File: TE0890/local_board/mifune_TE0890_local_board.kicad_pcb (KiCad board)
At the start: 2 copper layers, 139.7 x 120.7 mm, 76 parts, among them J1 Conn_01x01, J10 Conn_01x01, J11 Conn_01x01, J12 Conn_01x01, J13 1734035-1, J14 Conn_01x01, J15 Conn_01x01, J2 Conn_01x01, J3 Conn_01x01, J4 Conn_01x01, J5 Conn_01x01, J6 Conn_01x01, J7 Conn_01x01, J8 Conn_01x01, J9 Conn_01x01, U1 TE0890_80P, U2 TE0890_JTAG, U3 TE0790_Std, U4 TE0890_FTDI

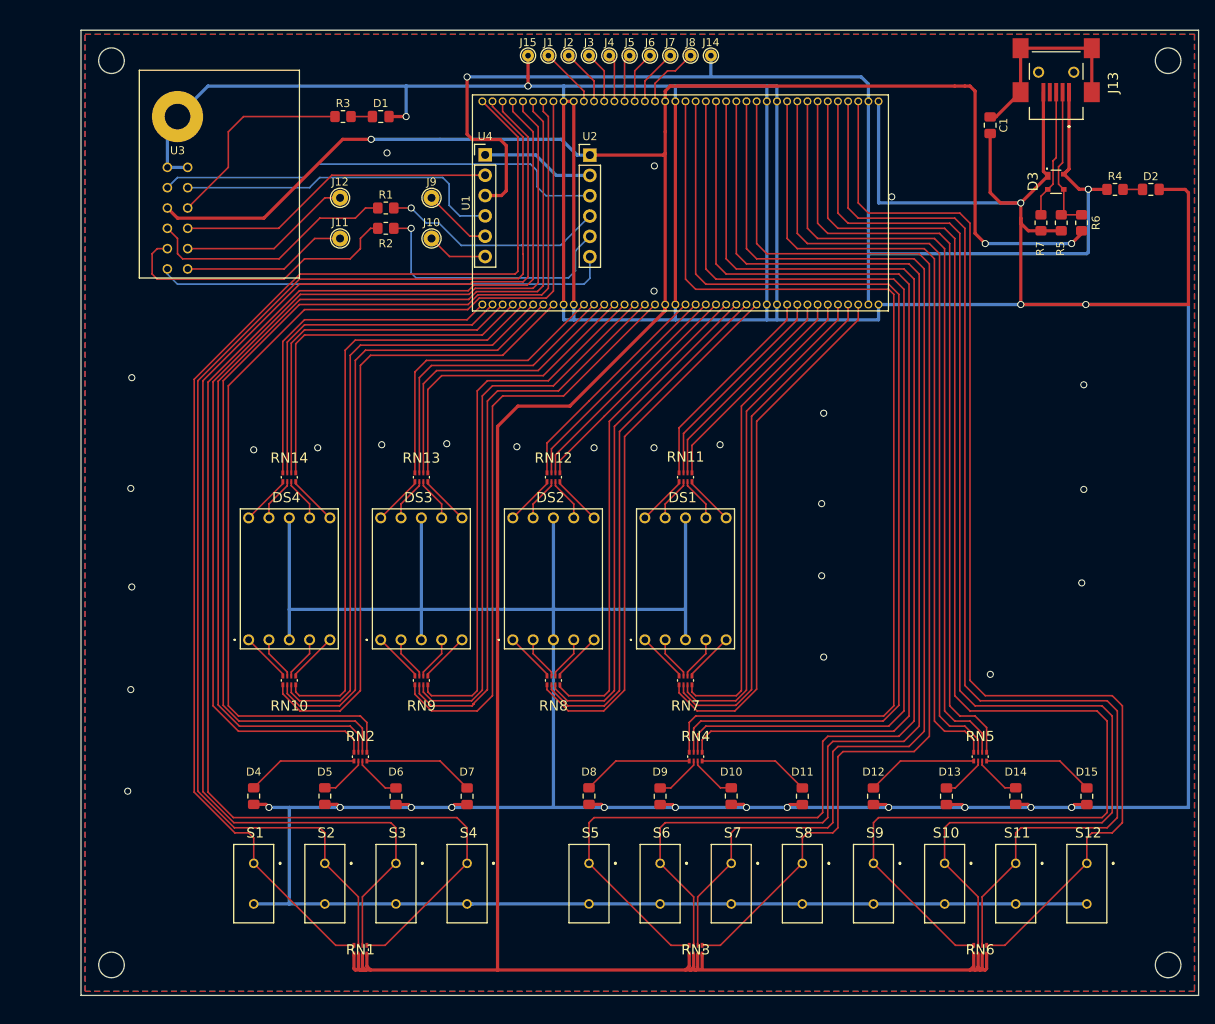
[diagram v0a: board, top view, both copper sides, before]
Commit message: local board rev.1.0 work in progress
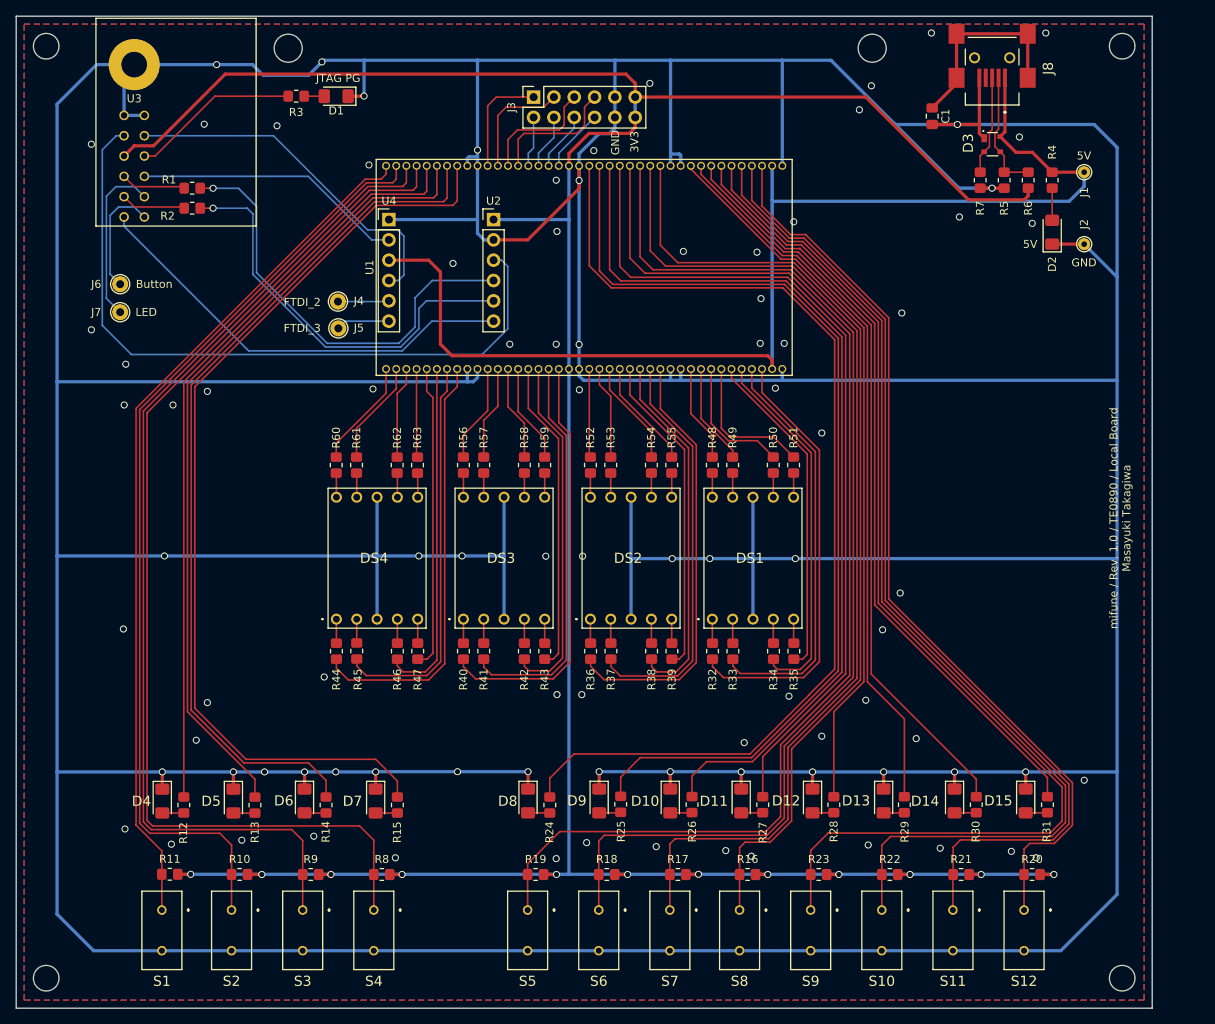
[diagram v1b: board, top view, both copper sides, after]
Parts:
- removed J10, J11, J12, J9: Conn_01x01, TestPoint:TestPoint_THTPad_D2.0mm_Drill1.0mm
- removed J13: 1734035-1, LibraryLoader:17340351
- removed J14, J15: Conn_01x01, TestPoint:TestPoint_THTPad_D1.5mm_Drill0.7mm
- removed RN1, RN10, RN11, RN12, RN13, RN14, RN2, RN3, RN4, RN5, RN6, RN7, RN8, RN9: EXB-N8V820JX, LibraryLoader:EXBN8V510JX
- added H5: MountingHole, MountingHole:MountingHole_3.5mm, F.Cu at (137.0, 34.0)
- added H6: MountingHole, MountingHole:MountingHole_3.5mm, F.Cu at (64.0, 34.0)
- added R10: 10k, Resistor_SMD:R_0805_2012Metric_Pad1.20x1.40mm_HandSolder, F.Cu at (57.9, 137.3)
- added R11: 10k, Resistor_SMD:R_0805_2012Metric_Pad1.20x1.40mm_HandSolder, F.Cu at (49.2, 137.3)
- added R12: 120, Resistor_SMD:R_0805_2012Metric_Pad1.20x1.40mm_HandSolder, F.Cu at (51.0, 128.6)
- added R13: 120, Resistor_SMD:R_0805_2012Metric_Pad1.20x1.40mm_HandSolder, F.Cu at (59.8, 128.6)
- added R14: 120, Resistor_SMD:R_0805_2012Metric_Pad1.20x1.40mm_HandSolder, F.Cu at (68.7, 128.6)
- added R15: 120, Resistor_SMD:R_0805_2012Metric_Pad1.20x1.40mm_HandSolder, F.Cu at (77.6, 128.6)
- added R16: 10k, Resistor_SMD:R_0805_2012Metric_Pad1.20x1.40mm_HandSolder, F.Cu at (121.4, 137.3)
- added R17: 10k, Resistor_SMD:R_0805_2012Metric_Pad1.20x1.40mm_HandSolder, F.Cu at (112.7, 137.3)
- added R18: 10k, Resistor_SMD:R_0805_2012Metric_Pad1.20x1.40mm_HandSolder, F.Cu at (103.8, 137.3)
- added R19: 10k, Resistor_SMD:R_0805_2012Metric_Pad1.20x1.40mm_HandSolder, F.Cu at (94.9, 137.3)
- added R20: 10k, Resistor_SMD:R_0805_2012Metric_Pad1.20x1.40mm_HandSolder, F.Cu at (157.0, 137.3)
- added R21: 10k, Resistor_SMD:R_0805_2012Metric_Pad1.20x1.40mm_HandSolder, F.Cu at (148.1, 137.3)
- added R22: 10k, Resistor_SMD:R_0805_2012Metric_Pad1.20x1.40mm_HandSolder, F.Cu at (139.2, 137.3)
- added R23: 10k, Resistor_SMD:R_0805_2012Metric_Pad1.20x1.40mm_HandSolder, F.Cu at (130.3, 137.3)
- added R24: 120, Resistor_SMD:R_0805_2012Metric_Pad1.20x1.40mm_HandSolder, F.Cu at (96.7, 128.6)
- added R25: 120, Resistor_SMD:R_0805_2012Metric_Pad1.20x1.40mm_HandSolder, F.Cu at (105.6, 128.5)
- added R26: 120, Resistor_SMD:R_0805_2012Metric_Pad1.20x1.40mm_HandSolder, F.Cu at (114.5, 128.5)
- added R27: 120, Resistor_SMD:R_0805_2012Metric_Pad1.20x1.40mm_HandSolder, F.Cu at (123.3, 128.6)
- added R28: 120, Resistor_SMD:R_0805_2012Metric_Pad1.20x1.40mm_HandSolder, F.Cu at (132.2, 128.6)
- added R29: 120, Resistor_SMD:R_0805_2012Metric_Pad1.20x1.40mm_HandSolder, F.Cu at (141.0, 128.6)
- added R30: 120, Resistor_SMD:R_0805_2012Metric_Pad1.20x1.40mm_HandSolder, F.Cu at (150.0, 128.6)
- added R31: 120, Resistor_SMD:R_0805_2012Metric_Pad1.20x1.40mm_HandSolder, F.Cu at (158.9, 128.6)
- added R32: 1.5k, Resistor_SMD:R_0805_2012Metric_Pad1.20x1.40mm_HandSolder, F.Cu at (117.0, 109.4)
- added R33: 1.5k, Resistor_SMD:R_0805_2012Metric_Pad1.20x1.40mm_HandSolder, F.Cu at (119.6, 109.4)
- added R34: 1.5k, Resistor_SMD:R_0805_2012Metric_Pad1.20x1.40mm_HandSolder, F.Cu at (124.7, 109.4)
- added R35: 1.5k, Resistor_SMD:R_0805_2012Metric_Pad1.20x1.40mm_HandSolder, F.Cu at (127.2, 109.4)
- added R36: 1.5k, Resistor_SMD:R_0805_2012Metric_Pad1.20x1.40mm_HandSolder, F.Cu at (101.8, 109.4)
- added R37: 1.5k, Resistor_SMD:R_0805_2012Metric_Pad1.20x1.40mm_HandSolder, F.Cu at (104.3, 109.4)
- added R38: 1.5k, Resistor_SMD:R_0805_2012Metric_Pad1.20x1.40mm_HandSolder, F.Cu at (109.4, 109.4)
- added R39: 1.5k, Resistor_SMD:R_0805_2012Metric_Pad1.20x1.40mm_HandSolder, F.Cu at (112.0, 109.4)
- added R40: 1.5k, Resistor_SMD:R_0805_2012Metric_Pad1.20x1.40mm_HandSolder, F.Cu at (85.9, 109.4)
- added R41: 1.5k, Resistor_SMD:R_0805_2012Metric_Pad1.20x1.40mm_HandSolder, F.Cu at (88.4, 109.4)
- added R42: 1.5k, Resistor_SMD:R_0805_2012Metric_Pad1.20x1.40mm_HandSolder, F.Cu at (93.5, 109.4)
- added R43: 1.5k, Resistor_SMD:R_0805_2012Metric_Pad1.20x1.40mm_HandSolder, F.Cu at (96.1, 109.4)
- added R44: 1.5k, Resistor_SMD:R_0805_2012Metric_Pad1.20x1.40mm_HandSolder, F.Cu at (70.0, 109.4)
- added R45: 1.5k, Resistor_SMD:R_0805_2012Metric_Pad1.20x1.40mm_HandSolder, F.Cu at (72.6, 109.4)
- added R46: 1.5k, Resistor_SMD:R_0805_2012Metric_Pad1.20x1.40mm_HandSolder, F.Cu at (77.6, 109.4)
- added R47: 1.5k, Resistor_SMD:R_0805_2012Metric_Pad1.20x1.40mm_HandSolder, F.Cu at (80.2, 109.4)
- added R48: 1.5k, Resistor_SMD:R_0805_2012Metric_Pad1.20x1.40mm_HandSolder, F.Cu at (117.0, 86.1)
- added R49: 1.5k, Resistor_SMD:R_0805_2012Metric_Pad1.20x1.40mm_HandSolder, F.Cu at (119.6, 86.1)
- added R50: 1.5k, Resistor_SMD:R_0805_2012Metric_Pad1.20x1.40mm_HandSolder, F.Cu at (124.6, 86.1)
- added R51: 1.5k, Resistor_SMD:R_0805_2012Metric_Pad1.20x1.40mm_HandSolder, F.Cu at (127.2, 86.1)
- added R52: 1.5k, Resistor_SMD:R_0805_2012Metric_Pad1.20x1.40mm_HandSolder, F.Cu at (101.8, 86.1)
- added R53: 1.5k, Resistor_SMD:R_0805_2012Metric_Pad1.20x1.40mm_HandSolder, F.Cu at (104.3, 86.1)
- added R54: 1.5k, Resistor_SMD:R_0805_2012Metric_Pad1.20x1.40mm_HandSolder, F.Cu at (109.4, 86.1)
- added R55: 1.5k, Resistor_SMD:R_0805_2012Metric_Pad1.20x1.40mm_HandSolder, F.Cu at (111.9, 86.1)
- added R56: 1.5k, Resistor_SMD:R_0805_2012Metric_Pad1.20x1.40mm_HandSolder, F.Cu at (85.9, 86.1)
- added R57: 1.5k, Resistor_SMD:R_0805_2012Metric_Pad1.20x1.40mm_HandSolder, F.Cu at (88.4, 86.1)
- added R58: 1.5k, Resistor_SMD:R_0805_2012Metric_Pad1.20x1.40mm_HandSolder, F.Cu at (93.5, 86.1)
- added R59: 1.5k, Resistor_SMD:R_0805_2012Metric_Pad1.20x1.40mm_HandSolder, F.Cu at (96.1, 86.1)
- added R60: 1.5k, Resistor_SMD:R_0805_2012Metric_Pad1.20x1.40mm_HandSolder, F.Cu at (70.0, 86.1)
- added R61: 1.5k, Resistor_SMD:R_0805_2012Metric_Pad1.20x1.40mm_HandSolder, F.Cu at (72.5, 86.1)
- added R62: 1.5k, Resistor_SMD:R_0805_2012Metric_Pad1.20x1.40mm_HandSolder, F.Cu at (77.6, 86.1)
- added R63: 1.5k, Resistor_SMD:R_0805_2012Metric_Pad1.20x1.40mm_HandSolder, F.Cu at (80.2, 86.1)
- added R8: 10k, Resistor_SMD:R_0805_2012Metric_Pad1.20x1.40mm_HandSolder, F.Cu at (75.7, 137.3)
- added R9: 10k, Resistor_SMD:R_0805_2012Metric_Pad1.20x1.40mm_HandSolder, F.Cu at (66.8, 137.3)
- D1, D10, D11, D12, D13, D14, D15, D2, D4, D5, D6, D7, D8, D9: footprint Capacitor_SMD:C_0805_2012Metric_Pad1.18x1.45mm_HandSolder -> LED_SMD:LED_1206_3216Metric_Pad1.42x1.75mm_HandSolder
- J3: value Conn_01x01 -> Conn_02x06_Top_Bottom; footprint TestPoint:TestPoint_THTPad_D1.5mm_Drill0.7mm -> Connector_PinSocket_2.54mm:PinSocket_2x06_P2.54mm_Vertical
- J4, J5, J6, J7: footprint TestPoint:TestPoint_THTPad_D1.5mm_Drill0.7mm -> TestPoint:TestPoint_THTPad_D2.0mm_Drill1.0mm
- J8: value Conn_01x01 -> 1734035-1; footprint TestPoint:TestPoint_THTPad_D1.5mm_Drill0.7mm -> LibraryLoader:17340351
- moved J7 75.9 mm to (43.0, 67.0)
- moved J6 72.1 mm to (43.0, 63.5)
- moved J2 68.6 mm to (163.5, 58.5)
- moved J1 68.5 mm to (163.5, 49.5)
- moved J5 49.9 mm to (70.3, 69.0)
- moved J4 45.8 mm to (70.2, 65.7)
- moved J8 37.8 mm to (152.0, 37.1), turned to -90 degrees
- moved R2 24.3 mm to (52.0, 54.0)
- moved R1 24.3 mm to (52.0, 51.5)
- moved U4 14.5 mm to (76.6, 55.4)
- moved U2 14.5 mm to (89.7, 55.4)
- moved U1 14.5 mm to (101.0, 61.4)
- moved D2 13.4 mm to (159.5, 57.0), turned to 90 degrees
- moved S2 13.0 mm to (56.9, 141.7)
- moved S3 13.0 mm to (65.8, 141.7)
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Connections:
- J1 pad 1: Net-(J1-Pad1) -> +5V
- J2 pad 1: Net-(J2-Pad1) -> GND
- J8 pad 1: Net-(J8-Pad1) -> +5V
- U1 pad 63: Net-(J8-Pad1) -> Net-(J3-Pad8)
- U1 pad 64: Net-(J7-Pad1) -> Net-(J3-Pad6)
- U1 pad 65: Net-(J6-Pad1) -> Net-(J3-Pad4)
- U1 pad 66: Net-(J5-Pad1) -> Net-(J3-Pad2)
- U1 pad 67: Net-(J4-Pad1) -> Net-(J3-Pad7)
- U1 pad 68: Net-(J3-Pad1) -> Net-(J3-Pad5)
- U1 pad 69: Net-(J2-Pad1) -> Net-(J3-Pad3)
- U1 pad 70: Net-(J1-Pad1) -> Net-(J3-Pad1)
- U3 pad 11: Net-(J11-Pad1) -> Net-(J6-Pad1)
- U3 pad 9: Net-(J12-Pad1) -> Net-(J7-Pad1)
- U4 pad 5: Net-(J9-Pad1) -> Net-(J4-Pad1)
- U4 pad 6: Net-(J10-Pad1) -> Net-(J5-Pad1)
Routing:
- net GND: track 901.7 -> 1107.5 mm, vias 42 -> 93
- net PSW0: track 150.6 -> 108.5 mm
- net PSW3: track 176.0 -> 137.1 mm
- net SLED3P: track 74.7 -> 38.1 mm
- net PSW1: track 154.5 -> 118.1 mm
- net LED8: track 130.7 -> 95.3 mm
- net PSW2: track 163.1 -> 127.7 mm
- net SLED3B: track 45.3 -> 11.1 mm
- net SLED3C: track 76.7 -> 43.1 mm
- net SLED3A: track 44.6 -> 11.5 mm
- net Net-(U2-Pad3): track 56.8 -> 88.8 mm
- net TSW4: track 172.1 -> 140.5 mm
- net LED9: track 130.9 -> 99.8 mm
- net SLED3F: track 43.9 -> 13.1 mm
- net TSW7: track 145.0 -> 114.5 mm
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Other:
- board size 139.7 x 120.7 mm -> 142 x 124 mm
- net class Default removed
- net class Power removed
- board text added: "3V3"
- board text added: "5V"
- board text added: "Button"
- board text added: "FTDI_2"
- board text added: "FTDI_3"
- board text added: "GND"
- board text added: "JTAG PG"
- board text added: "LED"
- board text added: "mifune / Rev. 1.0 / TE0890 / Local Board Masayuki Takagiwa"
